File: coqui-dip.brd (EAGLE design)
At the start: 100 x 80 mm, 14 parts, among them IC2 LM555D, IC3 LM555D, J1 AYZ0202

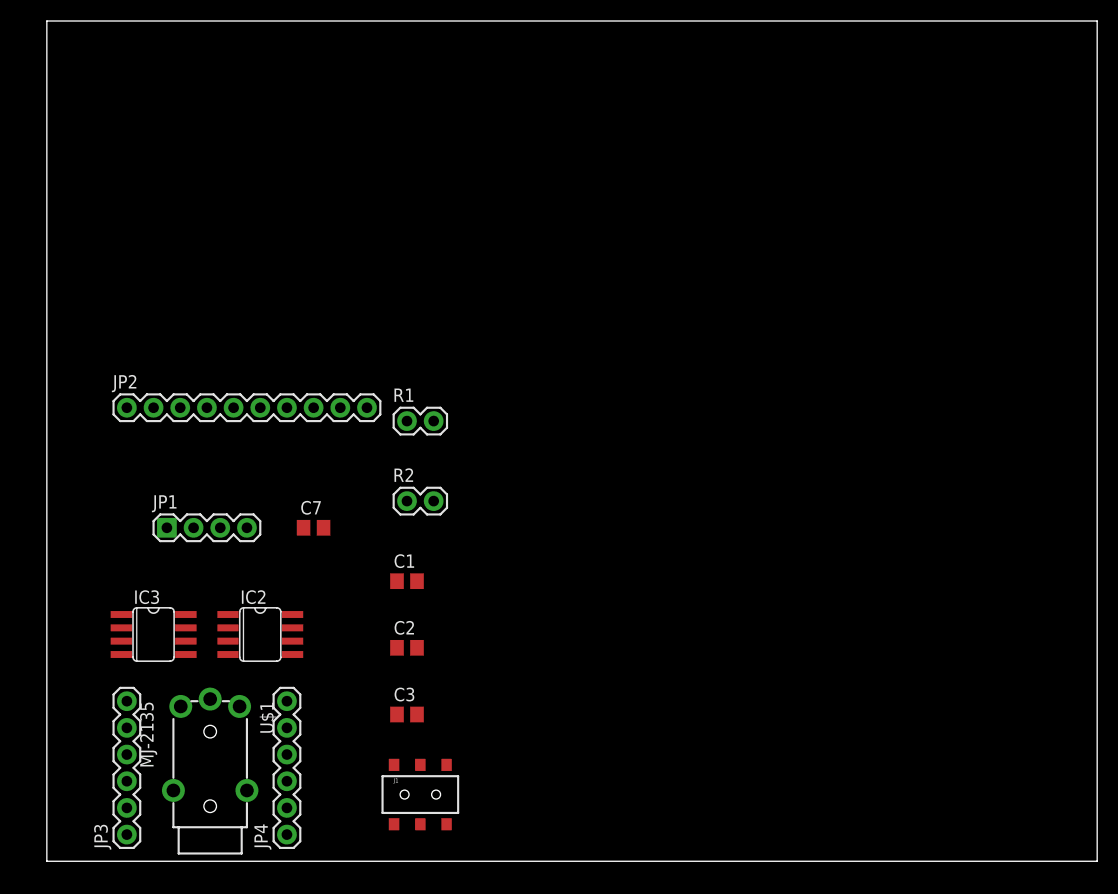
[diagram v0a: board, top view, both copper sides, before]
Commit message: update
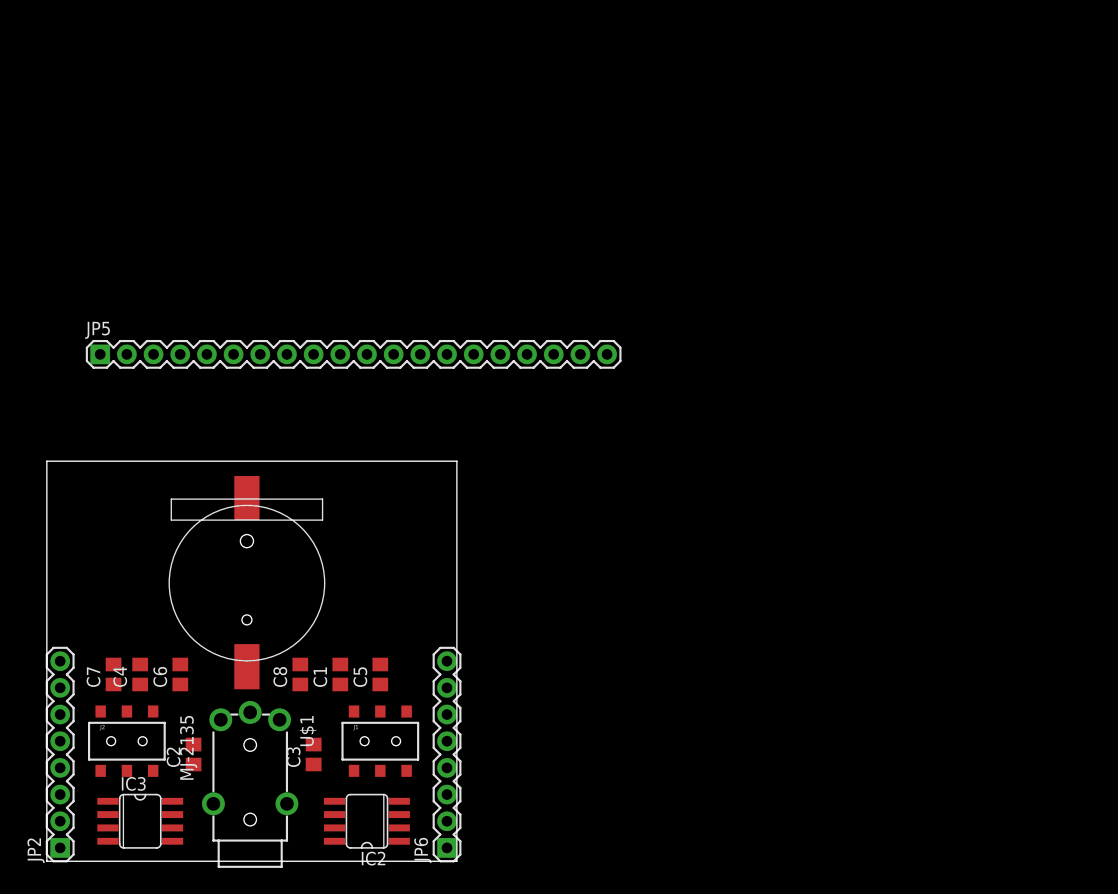
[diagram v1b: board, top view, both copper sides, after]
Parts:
- removed JP1: (no value), SparkFun-Connectors:1X04
- removed JP3, JP4: (no value), SparkFun-Connectors:1X06
- removed R1, R2: M02PTH, SparkFun-Connectors:1X02
- added BAT: CR1220, SparkFunNew:BATTCON_12MM_SMT
- added C4, C5, C6, C8: 0.1uF, rcl:C0805@1
- added J2: AYZ0202, SparkFunNew:AYZ0202
- added JP5: M20, SparkFun-Connectors:1X20
- added JP6: (no value), SparkFun-Connectors:1X08
- JP2: value M10" -> (none); device SparkFun-Connectors:1X10 -> SparkFun-Connectors:1X08
- moved JP2 42.4 mm to (1.27, 1.27), turned to 90 degrees
- moved C7 23.6 mm to (6.35, 17.8), turned to 90 degrees
- moved C2 22.7 mm to (14.0, 10.2), turned to 90 degrees
- moved IC2 20.5 mm to (30.5, 3.81), turned to 90 degrees
- moved IC3 17.8 mm to (8.89, 3.81)
- moved C1 10.9 mm to (27.9, 17.8), turned to 90 degrees
- moved C3 9.67 mm to (25.4, 10.2), turned to 90 degrees
- moved J1 6.35 mm to (31.8, 11.4)
- moved U$1 4.02 mm to (22.9, 14.0)
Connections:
- new net +: BAT.P$2
- new net GND1: BAT.P$1
- new net N$3: J2.3, J2.6
- new net VBAT1: J2.2, J2.5
- new net VDD1: J2.1, J2.4
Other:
- board size 100 x 80 mm -> 39 x 38.1 mm
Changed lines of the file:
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@@
 <board>
 <plain>
-<wire x1="0" y1="0" x2="100" y2="0" width="0" layer="20"/>
-<wire x1="100" y1="0" x2="100" y2="80" width="0" layer="20"/>
-<wire x1="100" y1="80" x2="0" y2="80" width="0" layer="20"/>
-<wire x1="0" y1="80" x2="0" y2="0" width="0" layer="20"/>
+<wire x1="0" y1="0" x2="39.04" y2="0" width="0" layer="20"/>
+<wire x1="39.04" y1="0" x2="39.04" y2="38.09" width="0" layer="20"/>
+<wire x1="39.04" y1="38.09" x2="0" y2="38.09" width="0" layer="20"/>
+<wire x1="0" y1="38.09" x2="0" y2="0" width="0" layer="20"/>
 </plain>
 <attributes>
@@
 </variantdefs>
 <classes>
-<class number="0" name="default" width="0.254" drill="0">
+<class number="0" name="default" width="0.2032" drill="0.3302">
 <clearance class="0" value="0.2032"/>
 </class>
@@
 </autorouter>
 <elements>
-<element name="U$1" library="iPhoneSoftModem" package="MJ-2135" value="MJ-2135" x="19.05" y="15.24" rot="R180"/>
-<element name="IC2" library="adafruit" package="SO08" value="LM555D" x="20.32" y="21.59" rot="R270"/>
-<element name="IC3" library="adafruit" package="SO08" value="LM555D" x="10.16" y="21.59" rot="R270"/>
-<element name="C7" library="rcl" package="C0805@1" value="0.1uF" x="25.4" y="31.75"/>
-<element name="R1" library="SparkFun-Connectors" package="1X02" value="M02PTH" x="34.29" y="41.91"/>
-<element name="R2" library="SparkFun-Connectors" package="1X02" value="M02PTH" x="34.29" y="34.29"/>
-<element name="C1" library="rcl" package="C0805@1" value="0.1uF" x="34.29" y="26.67"/>
-<element name="C2" library="rcl" package="C0805@1" value="0.01uF" x="34.29" y="20.32"/>
-<element name="C3" library="rcl" package="C0805@1" value="0.01uF" x="34.29" y="13.97"/>
-<element name="J1" library="SparkFunNew" package="AYZ0202" value="AYZ0202" x="35.56" y="6.35"/>
-<element name="JP3" library="SparkFun-Connectors" package="1X06" value="" x="7.62" y="2.54" rot="R90"/>
-<element name="JP4" library="SparkFun-Connectors" package="1X06" value="" x="22.86" y="2.54" rot="R90"/>
-<element name="JP1" library="SparkFun-Connectors" package="1X04" value="" x="11.43" y="31.75"/>
-<element name="JP2" library="SparkFun-Connectors" package="1X10" value="M10&quot;" x="7.62" y="43.18"/>
+<element name="U$1" library="iPhoneSoftModem" package="MJ-2135" value="MJ-2135" x="22.86" y="13.97" rot="R180"/>
+<element name="IC2" library="adafruit" package="SO08" value="LM555D" x="30.48" y="3.81" rot="R90"/>
+<element name="IC3" library="adafruit" package="SO08" value="LM555D" x="8.89" y="3.81" rot="R270"/>
+<element name="C7" library="rcl" package="C0805@1" value="0.1uF" x="6.35" y="17.78" rot="R90"/>
+<element name="C1" library="rcl" package="C0805@1" value="0.1uF" x="27.94" y="17.78" rot="R90"/>
+<element name="C2" library="rcl" package="C0805@1" value="0.01uF" x="13.97" y="10.16" rot="R90"/>
+<element name="C3" library="rcl" package="C0805@1" value="0.01uF" x="25.4" y="10.16" rot="R90"/>
+<element name="J1" library="SparkFunNew" package="AYZ0202" value="AYZ0202" x="31.75" y="11.43"/>
+<element name="JP5" library="SparkFun-Connectors" package="1X20" value="M20" x="5.08" y="48.26"/>
+<element name="JP2" library="SparkFun-Connectors" package="1X08" value="" x="1.27" y="1.27" rot="R90"/>
+<element name="JP6" library="SparkFun-Connectors" package="1X08" value="" x="38.1" y="1.27" rot="R90"/>
+<element name="C4" library="rcl" package="C0805@1" value="0.1uF" x="8.89" y="17.78" rot="R90"/>
+<element name="C5" library="rcl" package="C0805@1" value="0.1uF" x="31.75" y="17.78" rot="R90"/>
+<element name="J2" library="SparkFunNew" package="AYZ0202" value="AYZ0202" x="7.62" y="11.43"/>
+<element name="BAT" library="SparkFunNew" package="BATTCON_12MM_SMT" value="CR1220" x="19.05" y="30.48" rot="R180"/>
+<element name="C6" library="rcl" package="C0805@1" value="0.1uF" x="12.7" y="17.78" rot="R90"/>
+<element name="C8" library="rcl" package="C0805@1" value="0.1uF" x="24.13" y="17.78" rot="R90"/>
 </elements>
 <signals>
@@
 <contactref element="IC2" pad="1"/>
 <contactref element="IC3" pad="1"/>
-<wire x1="7.0866" y1="23.495" x2="17.2466" y2="23.495" width="0" layer="19" extent="1-1"/>
-<wire x1="12.75" y1="14.74" x2="7.0866" y2="23.495" width="0" layer="19" extent="1-1"/>
+<wire x1="5.8166" y1="5.715" x2="33.5534" y2="1.905" width="0" layer="19" extent="1-1"/>
+<wire x1="16.56" y1="13.47" x2="5.8166" y2="5.715" width="0" layer="19" extent="1-1"/>
 </signal>
 <signal name="N$6">
@@
 <contactref element="IC2" pad="8"/>
 <contactref element="IC3" pad="8"/>
-<wire x1="13.2334" y1="23.495" x2="23.3934" y2="23.495" width="0" layer="19" extent="1-1"/>
+<wire x1="11.9634" y1="5.715" x2="27.4066" y2="1.905" width="0" layer="19" extent="1-1"/>
 </signal>
 <signal name="VDD">
 <contactref element="J1" pad="1"/>
 <contactref element="J1" pad="4"/>
-<wire x1="33.06" y1="9.175" x2="33.06" y2="3.525" width="0" layer="19" extent="1-1"/>
+<wire x1="29.25" y1="14.255" x2="29.25" y2="8.605" width="0" layer="19" extent="1-1"/>
 </signal>
 <signal name="VBAT">
 <contactref element="J1" pad="2"/>
 <contactref element="J1" pad="5"/>
-<wire x1="35.56" y1="9.175" x2="35.56" y2="3.525" width="0" layer="19" extent="1-1"/>
+<wire x1="31.75" y1="14.255" x2="31.75" y2="8.605" width="0" layer="19" extent="1-1"/>
 </signal>
 <signal name="N$2">
 <contactref element="J1" pad="3"/>
 <contactref element="J1" pad="6"/>
-<wire x1="38.06" y1="9.175" x2="38.06" y2="3.525" width="0" layer="19" extent="1-1"/>
+<wire x1="34.25" y1="14.255" x2="34.25" y2="8.605" width="0" layer="19" extent="1-1"/>
+</signal>
+<signal name="VDD1">
+<contactref element="J2" pad="1"/>
+<contactref element="J2" pad="4"/>
+<wire x1="5.12" y1="14.255" x2="5.12" y2="8.605" width="0" layer="19" extent="1-1"/>
+</signal>
+<signal name="VBAT1">
+<contactref element="J2" pad="2"/>
+<contactref element="J2" pad="5"/>
+<wire x1="7.62" y1="14.255" x2="7.62" y2="8.605" width="0" layer="19" extent="1-1"/>
+</signal>
+<signal name="N$3">
+<contactref element="J2" pad="3"/>
+<contactref element="J2" pad="6"/>
+<wire x1="10.12" y1="14.255" x2="10.12" y2="8.605" width="0" layer="19" extent="1-1"/>
+</signal>
+<signal name="+">
+<contactref element="BAT" pad="P$2"/>
+</signal>
+<signal name="GND1">
+<contactref element="BAT" pad="P$1"/>
 </signal>
 </signals>
